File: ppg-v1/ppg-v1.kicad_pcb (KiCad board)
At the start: 2 copper layers, 31 x 36.6 mm, 56 parts, among them J1 USB_microB_2040002-1, J2 Conn_01x04_Male, SW1 SW_Push, SW2 SW_Push, SW3 PCM12, U1 STM32F411CEUx, U2 MCP73831T-2ACI/OT, U3 Opamp_Dual_Generic, U4 Opamp_Dual_Generic, U5 TPS2113APW, U6 MCP1702T-3302E/CB, U7 BM71BLES1FC2, Y1 12MHz, Y2 32K768

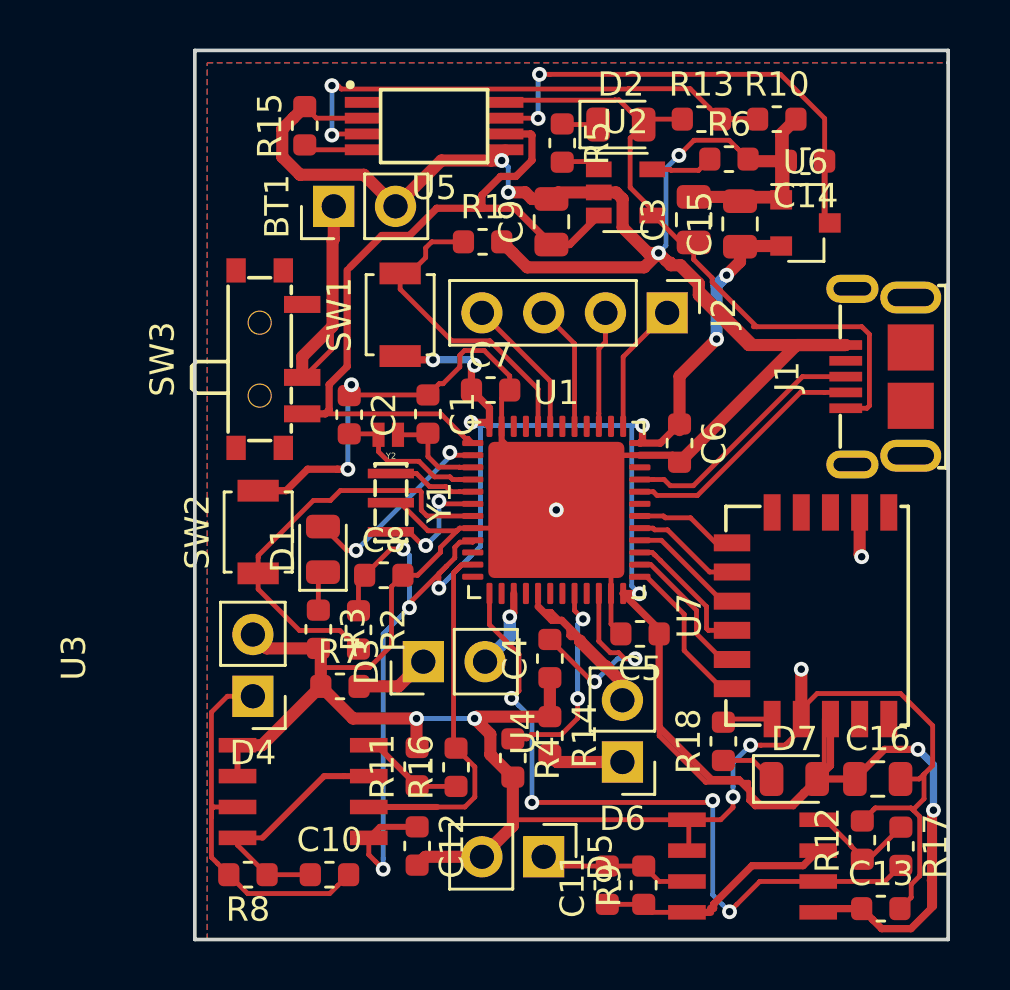
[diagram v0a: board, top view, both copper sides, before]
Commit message: fix fills
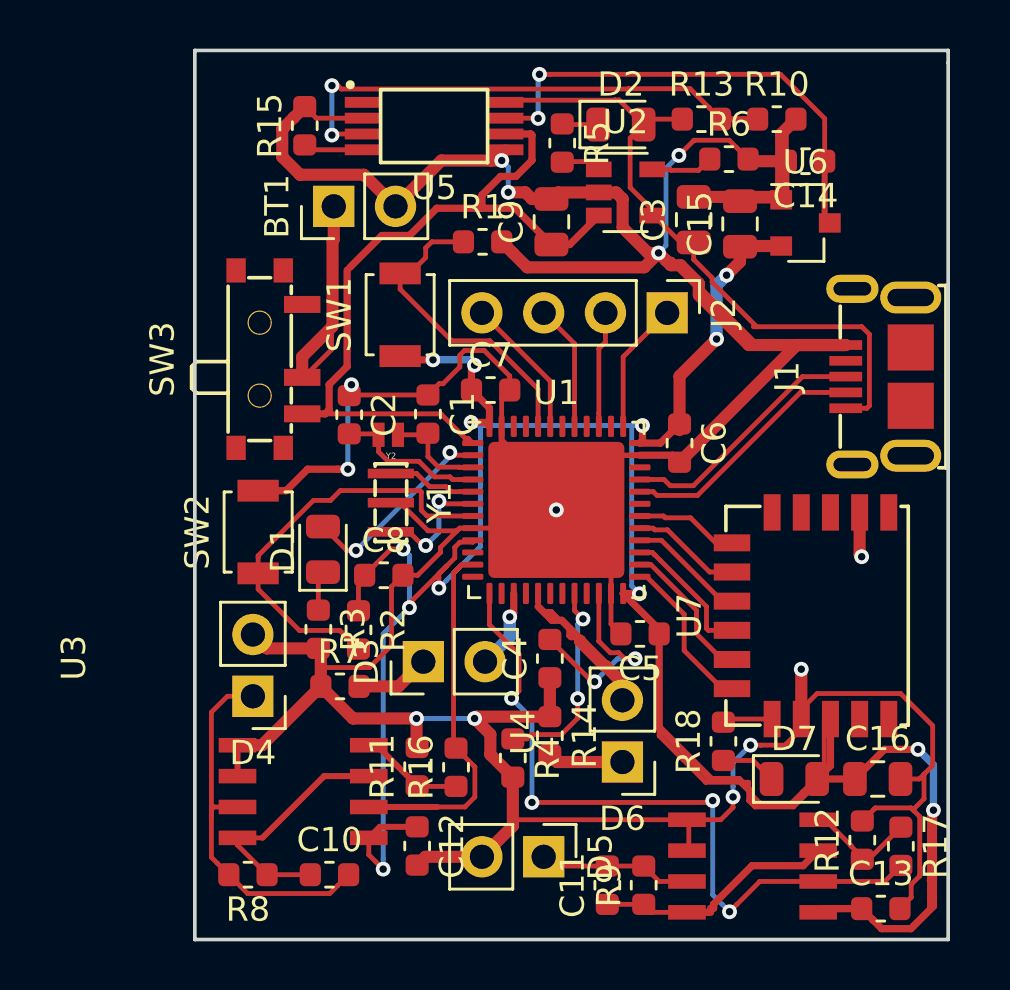
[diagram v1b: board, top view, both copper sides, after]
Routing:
- added copper zone on F.Cu, net +3V3
- removed copper zone on F.Cu, net (none)
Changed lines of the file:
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@@
     (47 F.CrtYd user)
     (48 B.Fab user)
-    (49 F.Fab user)
+    (49 F.Fab user hide)
   )
   (setup
@@
   (segment (start 193.802 107.0285) (end 193.402 107.0285) (width 0.2) (layer F.Cu) (net 78))
   (segment (start 193.402 107.0285) (end 191.8335 105.46) (width 0.2) (layer F.Cu) (net 78))
-  (zone (net 0) (net_name "") (layer F.Cu) (hatch edge 0.508)
+  (zone (net 7) (net_name +3V3) (layer F.Cu) (hatch edge 0.508)
     (connect_pads (clearance 0.508))
     (min_thickness 0.254)
-    (fill yes (arc_segments 16) (thermal_gap 0.508) (thermal_bridge_width 0.508))
+    (fill yes (arc_segments 32) (thermal_gap 0.508) (thermal_bridge_width 0.508))
     (polygon
       (pts
-        (xy 172.212 81.28) (xy 202.692 81.28) (xy 202.692 117.348) (xy 172.212 117.348)
+        (xy 202.692 80.772) (xy 202.692 117.348) (xy 171.704 117.348) (xy 171.704 80.772)
       )
     )
@@
     (connect_pads (clearance 0.508))
     (min_thickness 0.254)
-    (fill yes (arc_segments 16) (thermal_gap 0.508) (thermal_bridge_width 0.508))
+    (fill yes (arc_segments 32) (thermal_gap 0.508) (thermal_bridge_width 0.508))
     (polygon
       (pts
-        (xy 172.212 81.28) (xy 202.692 81.28) (xy 202.692 117.348) (xy 172.212 117.348)
+        (xy 202.692 80.772) (xy 202.692 117.348) (xy 171.704 117.348) (xy 171.704 80.772)
       )
     )

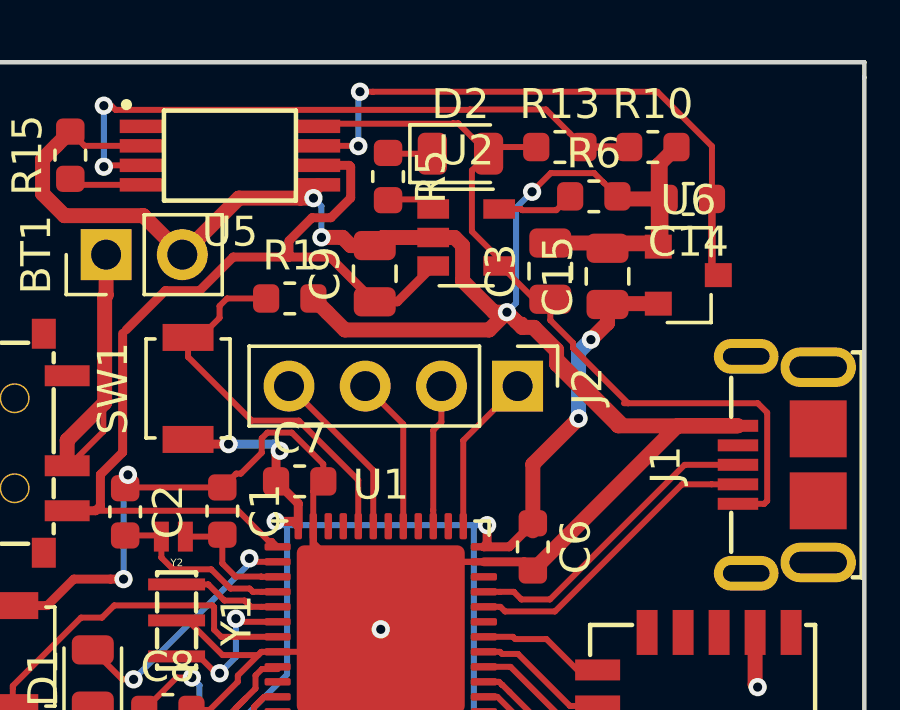
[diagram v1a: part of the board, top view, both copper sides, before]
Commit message: small fixes
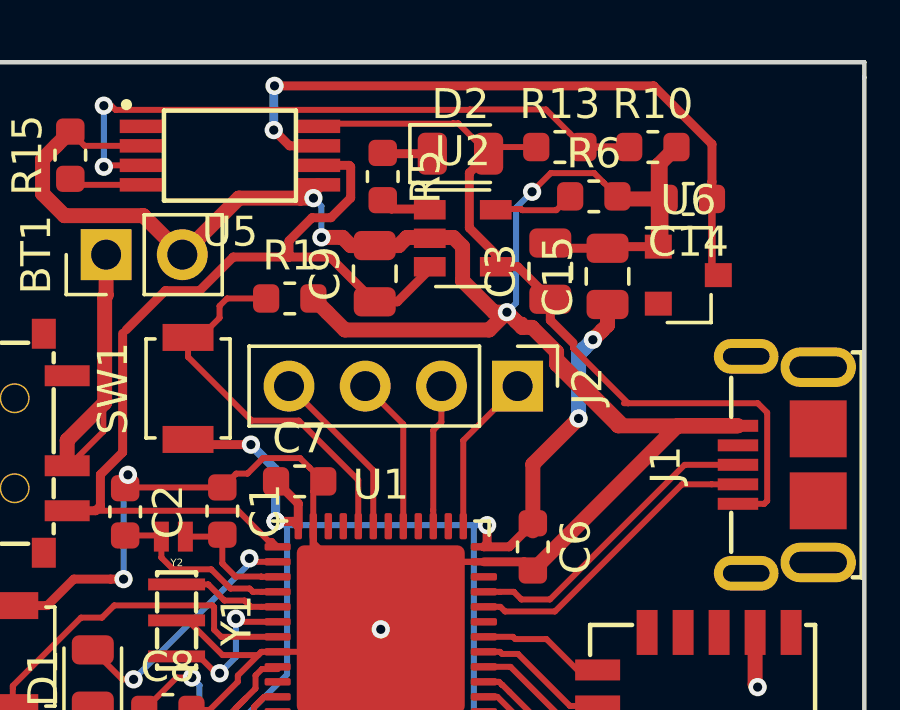
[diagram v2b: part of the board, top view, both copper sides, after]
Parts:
- moved R5 0.18 mm to (186.6, 84.6)
- moved U2 0.12 mm to (189.3, 86.6)
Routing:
- net GND: track 227.8 -> 222.8 mm
- net Net-(C14-Pad1): track 20.0 -> 23.0 mm
- net +3V3: track 129.8 -> 128.9 mm
